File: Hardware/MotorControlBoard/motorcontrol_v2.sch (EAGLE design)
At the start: 26 parts, among them U1 ATMEGA328P-AU

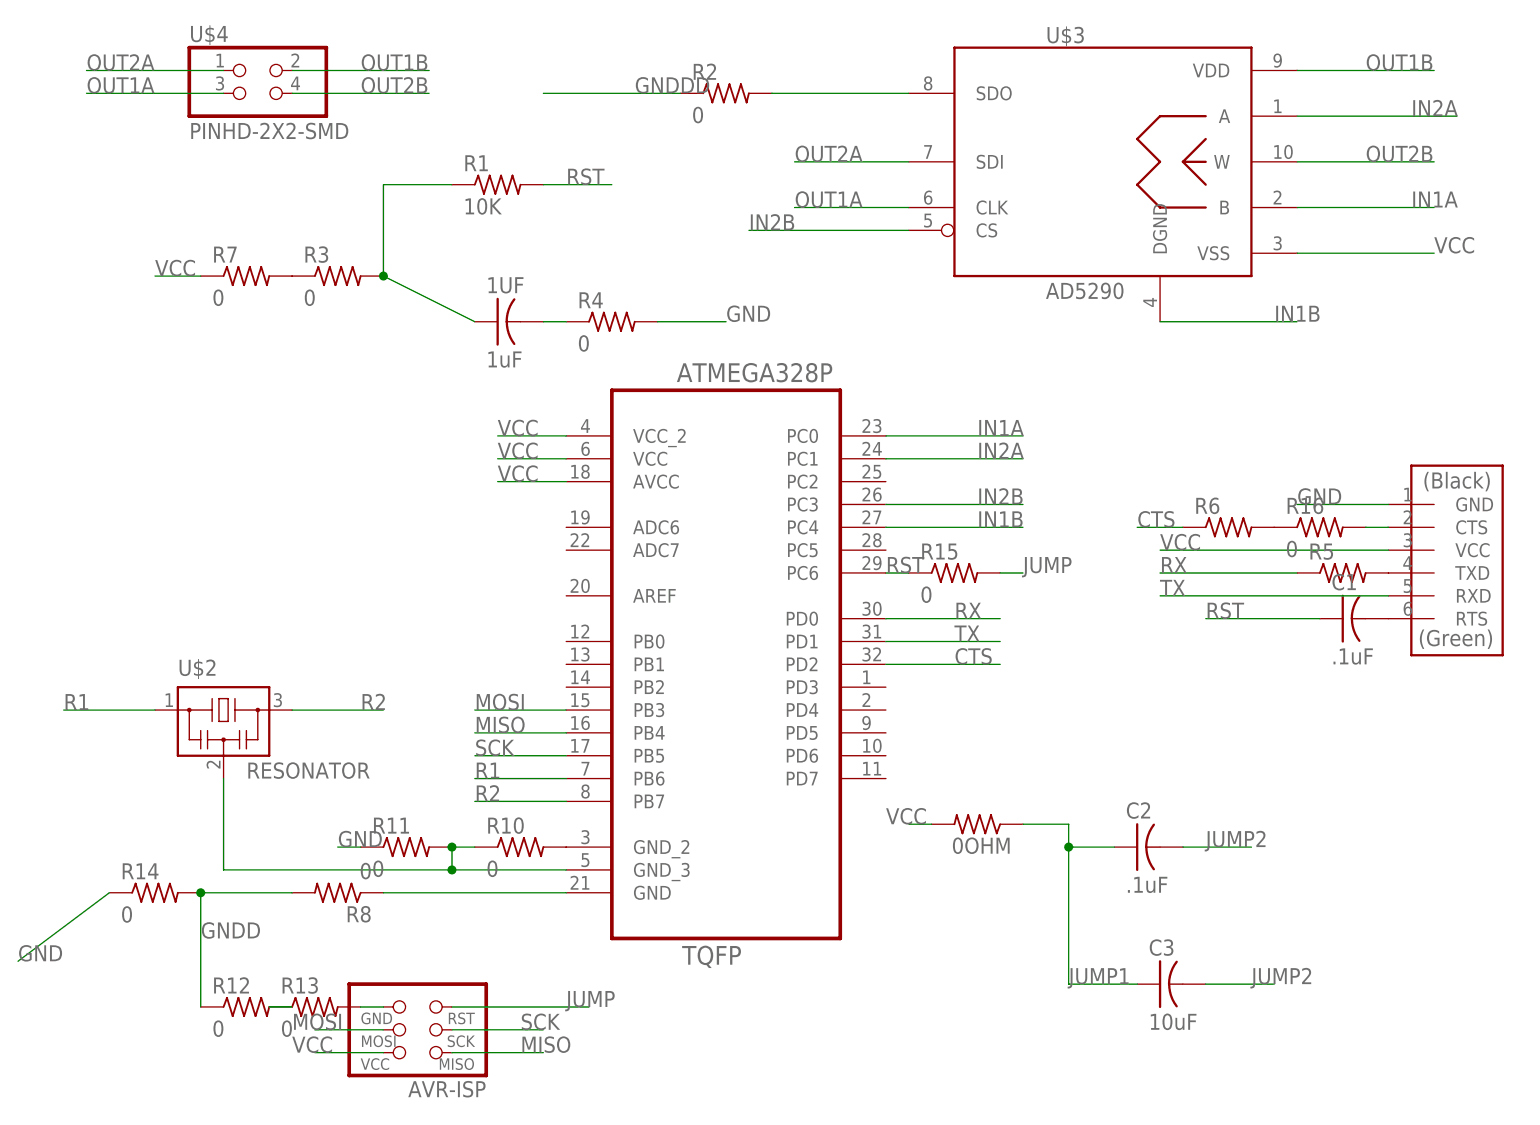
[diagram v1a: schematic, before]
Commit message: new board stuff
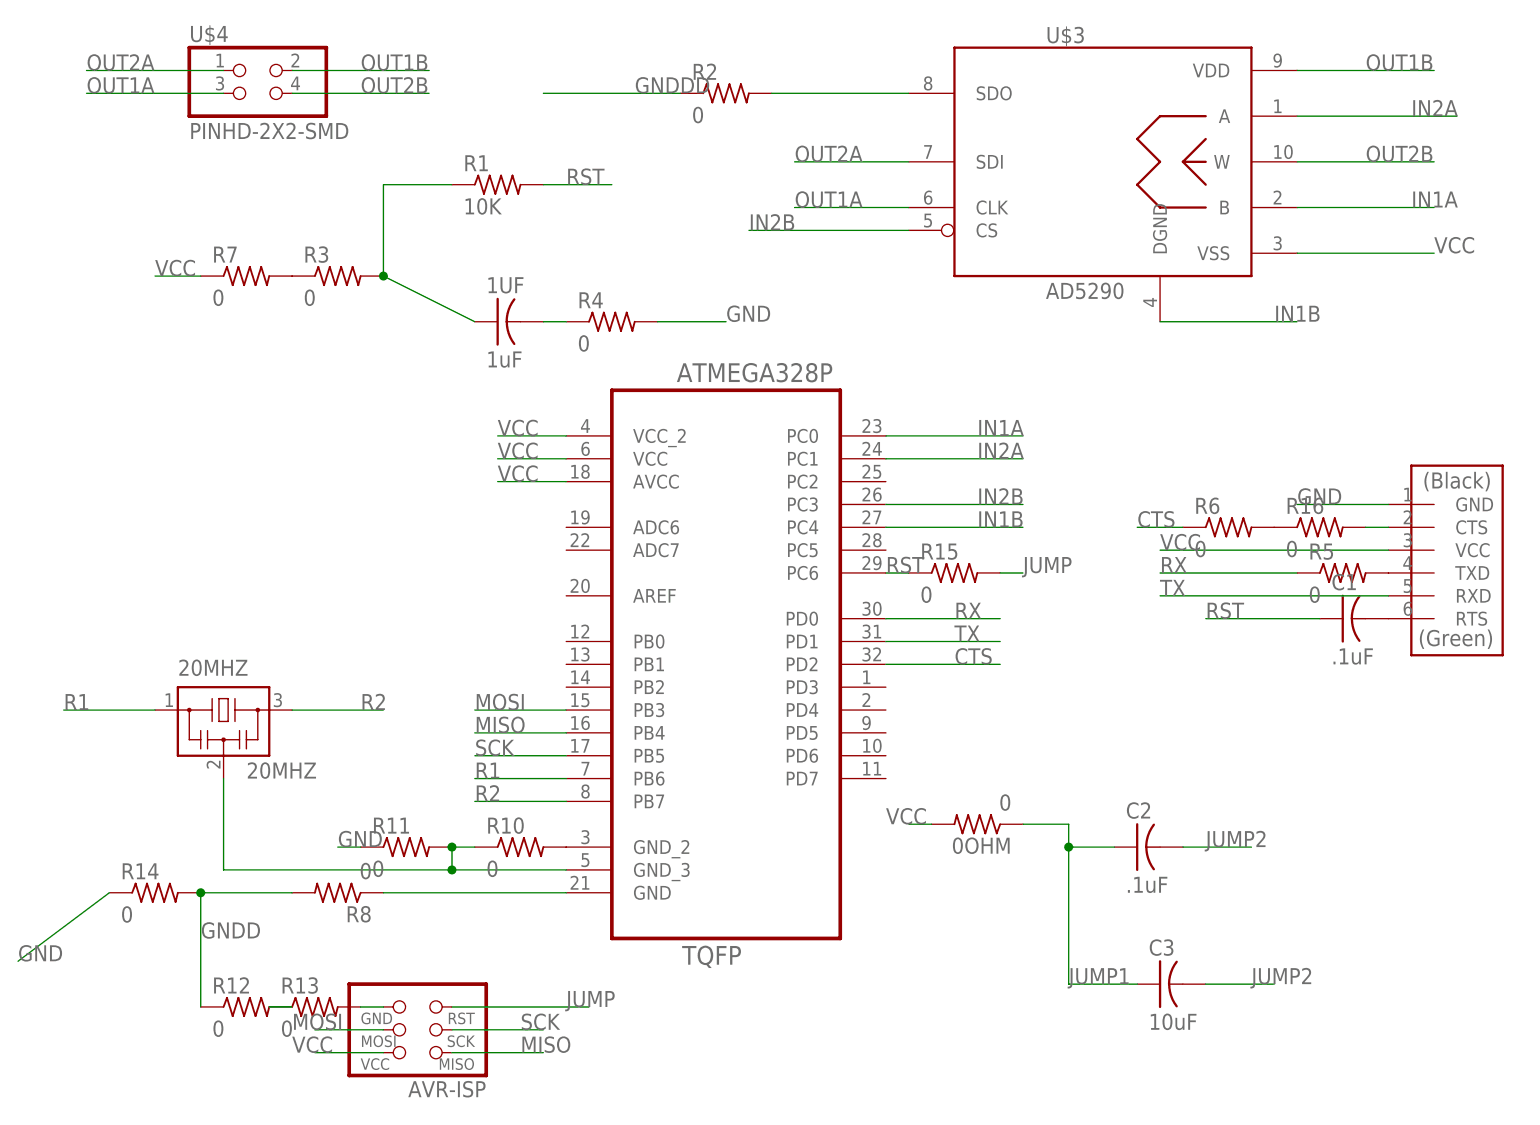
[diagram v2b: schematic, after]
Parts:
- 0OHM, R5, R6: value (none) -> 0
- 20MHZ: value RESONATOR -> 20MHZ
- renumbered U$2 to 20MHZ
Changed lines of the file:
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@@
 <part name="U1" library="fab" deviceset="ATMEGA328P-AU" device=""/>
 <part name="U$1" library="fab" deviceset="FTDI-SMD-HEADER" device=""/>
-<part name="U$2" library="fab" deviceset="RESONATOR" device=""/>
+<part name="20MHZ" library="fab" deviceset="RESONATOR" device="" value="20MHZ"/>
 <part name="AVR-ISP" library="fab" deviceset="AVRISP" device="SMD" value=""/>
 <part name="1UF" library="fab" deviceset="CAP-US" device="1206FAB" value="1uF"/>
@@
 <part name="U$3" library="BillPorter" deviceset="AD5290" device=""/>
 <part name="U$4" library="fab" deviceset="PINHD-2X2-SMD" device=""/>
-<part name="0OHM" library="fab" deviceset="RES-US" device="1206FAB"/>
+<part name="0OHM" library="fab" deviceset="RES-US" device="1206FAB" value="0"/>
 <part name="R2" library="fab" deviceset="RES-US" device="1206FAB" value="0"/>
 <part name="R4" library="fab" deviceset="RES-US" device="1206FAB" value="0"/>
@@
 <part name="R16" library="fab" deviceset="RES-US" device="1206FAB" value="0"/>
 <part name="C1" library="fab" deviceset="CAP-US" device="1206FAB" value=".1uF"/>
-<part name="R5" library="fab" deviceset="RES-US" device="1206FAB"/>
-<part name="R6" library="fab" deviceset="RES-US" device="1206FAB"/>
+<part name="R5" library="fab" deviceset="RES-US" device="1206FAB" value="0"/>
+<part name="R6" library="fab" deviceset="RES-US" device="1206FAB" value="0"/>
 <part name="R3" library="fab" deviceset="RES-US" device="1206FAB" value="0"/>
 <part name="R7" library="fab" deviceset="RES-US" device="1206FAB" value="0"/>
@@
 <instance part="U1" gate="A" x="76.2" y="53.34"/>
 <instance part="U$1" gate="G$1" x="149.86" y="55.88"/>
-<instance part="U$2" gate="G$1" x="20.32" y="45.72"/>
+<instance part="20MHZ" gate="G$1" x="20.32" y="45.72"/>
 <instance part="AVR-ISP" gate="G$1" x="43.18" y="10.16" rot="R180"/>
 <instance part="1UF" gate="G$1" x="50.8" y="88.9"/>
@@
 </segment>
 <segment>
-<pinref part="U$2" gate="G$1" pin="1"/>
+<pinref part="20MHZ" gate="G$1" pin="1"/>
 <wire x1="12.7" y1="45.72" x2="2.54" y2="45.72" width="0.1524" layer="91"/>
 <label x="2.54" y="45.72" size="1.778" layer="95"/>
@@
 </segment>
 <segment>
-<pinref part="U$2" gate="G$1" pin="3"/>
+<pinref part="20MHZ" gate="G$1" pin="3"/>
 <wire x1="27.94" y1="45.72" x2="38.1" y2="45.72" width="0.1524" layer="91"/>
 <label x="35.56" y="45.72" size="1.778" layer="95"/>
@@
 <wire x1="45.72" y1="27.94" x2="45.72" y2="30.48" width="0.1524" layer="91"/>
 <junction x="45.72" y="30.48"/>
-<pinref part="U$2" gate="G$1" pin="2"/>
+<pinref part="20MHZ" gate="G$1" pin="2"/>
 <wire x1="20.32" y1="38.1" x2="20.32" y2="27.94" width="0.1524" layer="91"/>
 <wire x1="20.32" y1="27.94" x2="45.72" y2="27.94" width="0.1524" layer="91"/>

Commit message: lots of changes
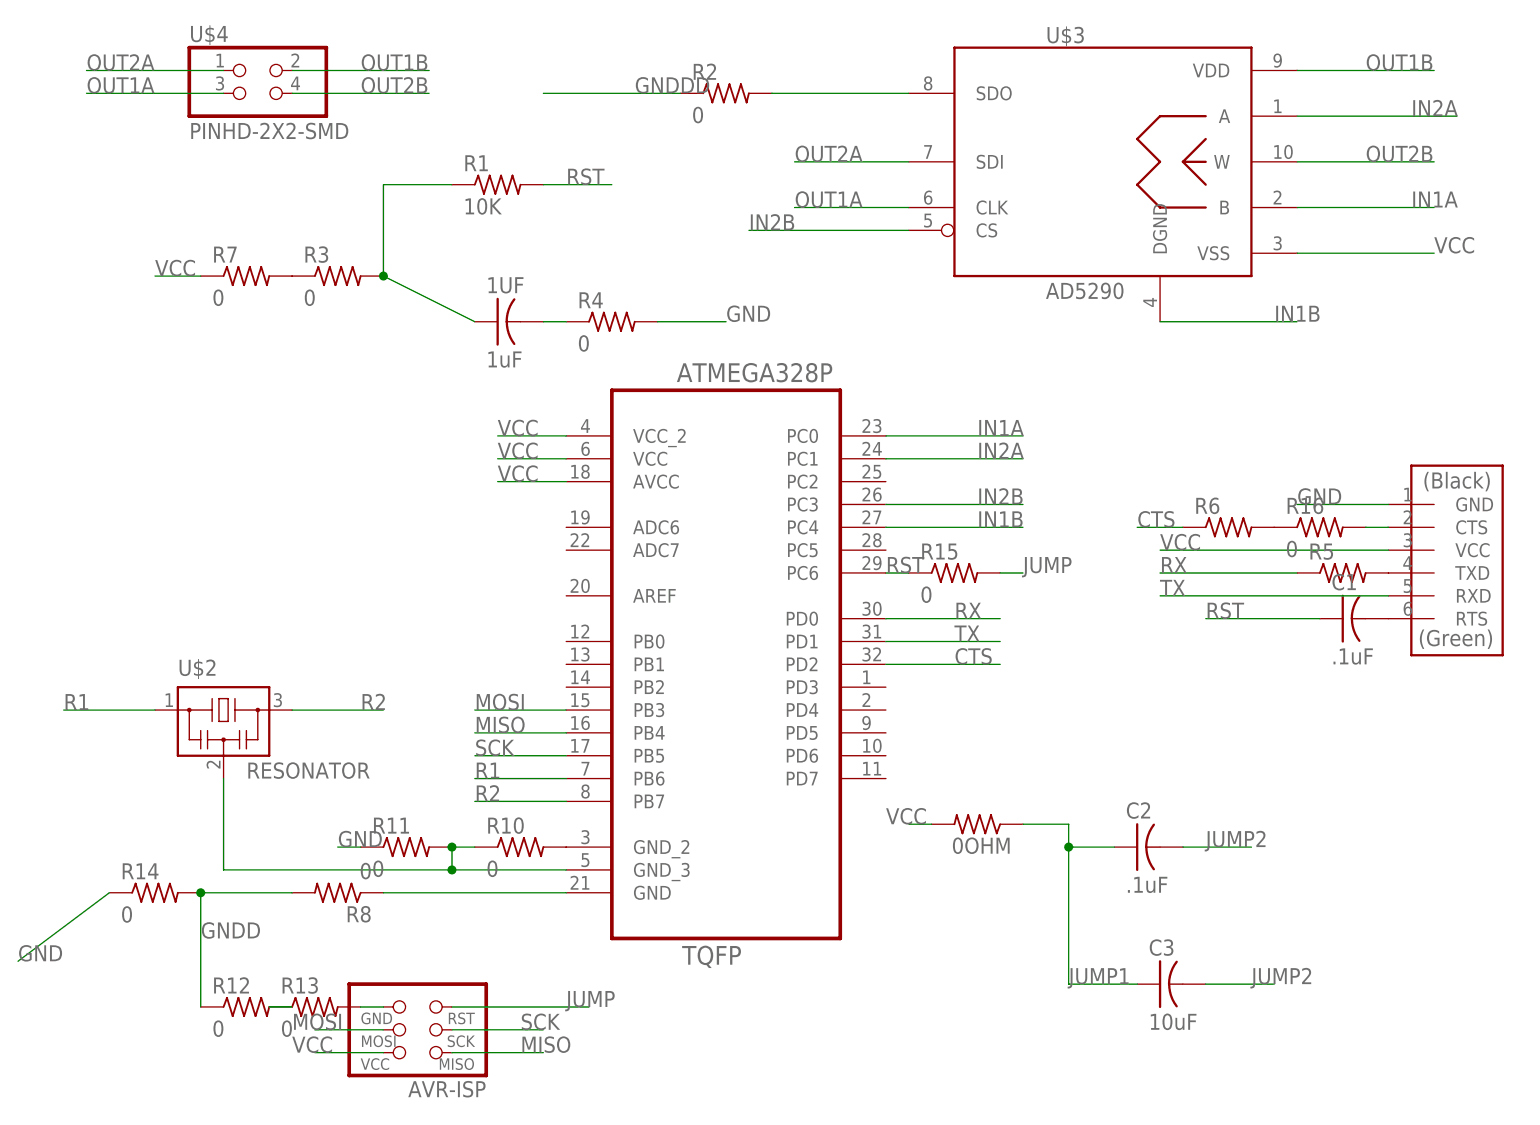
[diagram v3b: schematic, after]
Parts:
- 0OHM, R5, R6: value 0 -> (none)
- U$2: value 20MHZ -> RESONATOR
- renumbered 20MHZ to U$2
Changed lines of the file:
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@@
 <part name="U1" library="fab" deviceset="ATMEGA328P-AU" device=""/>
 <part name="U$1" library="fab" deviceset="FTDI-SMD-HEADER" device=""/>
-<part name="20MHZ" library="fab" deviceset="RESONATOR" device="" value="20MHZ"/>
+<part name="U$2" library="fab" deviceset="RESONATOR" device=""/>
 <part name="AVR-ISP" library="fab" deviceset="AVRISP" device="SMD" value=""/>
 <part name="1UF" library="fab" deviceset="CAP-US" device="1206FAB" value="1uF"/>
@@
 <part name="U$3" library="BillPorter" deviceset="AD5290" device=""/>
 <part name="U$4" library="fab" deviceset="PINHD-2X2-SMD" device=""/>
-<part name="0OHM" library="fab" deviceset="RES-US" device="1206FAB" value="0"/>
+<part name="0OHM" library="fab" deviceset="RES-US" device="1206FAB"/>
 <part name="R2" library="fab" deviceset="RES-US" device="1206FAB" value="0"/>
 <part name="R4" library="fab" deviceset="RES-US" device="1206FAB" value="0"/>
@@
 <part name="R16" library="fab" deviceset="RES-US" device="1206FAB" value="0"/>
 <part name="C1" library="fab" deviceset="CAP-US" device="1206FAB" value=".1uF"/>
-<part name="R5" library="fab" deviceset="RES-US" device="1206FAB" value="0"/>
-<part name="R6" library="fab" deviceset="RES-US" device="1206FAB" value="0"/>
+<part name="R5" library="fab" deviceset="RES-US" device="1206FAB"/>
+<part name="R6" library="fab" deviceset="RES-US" device="1206FAB"/>
 <part name="R3" library="fab" deviceset="RES-US" device="1206FAB" value="0"/>
 <part name="R7" library="fab" deviceset="RES-US" device="1206FAB" value="0"/>
@@
 <instance part="U1" gate="A" x="76.2" y="53.34"/>
 <instance part="U$1" gate="G$1" x="149.86" y="55.88"/>
-<instance part="20MHZ" gate="G$1" x="20.32" y="45.72"/>
+<instance part="U$2" gate="G$1" x="20.32" y="45.72"/>
 <instance part="AVR-ISP" gate="G$1" x="43.18" y="10.16" rot="R180"/>
 <instance part="1UF" gate="G$1" x="50.8" y="88.9"/>
@@
 </segment>
 <segment>
-<pinref part="20MHZ" gate="G$1" pin="1"/>
+<pinref part="U$2" gate="G$1" pin="1"/>
 <wire x1="12.7" y1="45.72" x2="2.54" y2="45.72" width="0.1524" layer="91"/>
 <label x="2.54" y="45.72" size="1.778" layer="95"/>
@@
 </segment>
 <segment>
-<pinref part="20MHZ" gate="G$1" pin="3"/>
+<pinref part="U$2" gate="G$1" pin="3"/>
 <wire x1="27.94" y1="45.72" x2="38.1" y2="45.72" width="0.1524" layer="91"/>
 <label x="35.56" y="45.72" size="1.778" layer="95"/>
@@
 <wire x1="45.72" y1="27.94" x2="45.72" y2="30.48" width="0.1524" layer="91"/>
 <junction x="45.72" y="30.48"/>
-<pinref part="20MHZ" gate="G$1" pin="2"/>
+<pinref part="U$2" gate="G$1" pin="2"/>
 <wire x1="20.32" y1="38.1" x2="20.32" y2="27.94" width="0.1524" layer="91"/>
 <wire x1="20.32" y1="27.94" x2="45.72" y2="27.94" width="0.1524" layer="91"/>
